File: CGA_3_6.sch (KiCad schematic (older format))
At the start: 1 part, among them U4 74S174

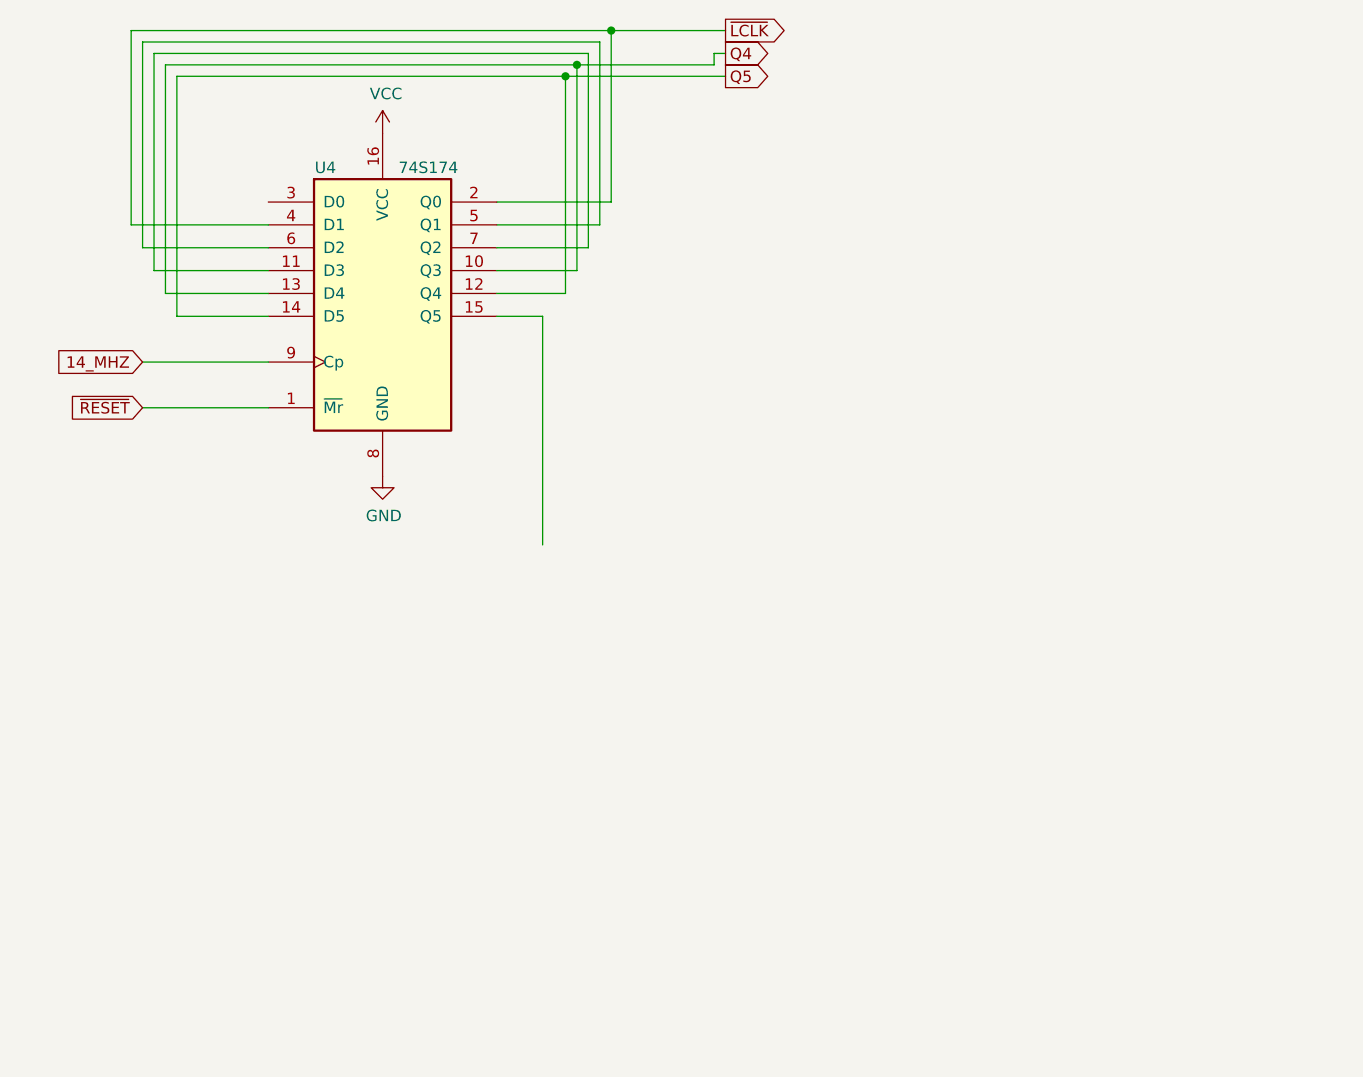
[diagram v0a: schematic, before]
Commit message: More sheet 3 drawing
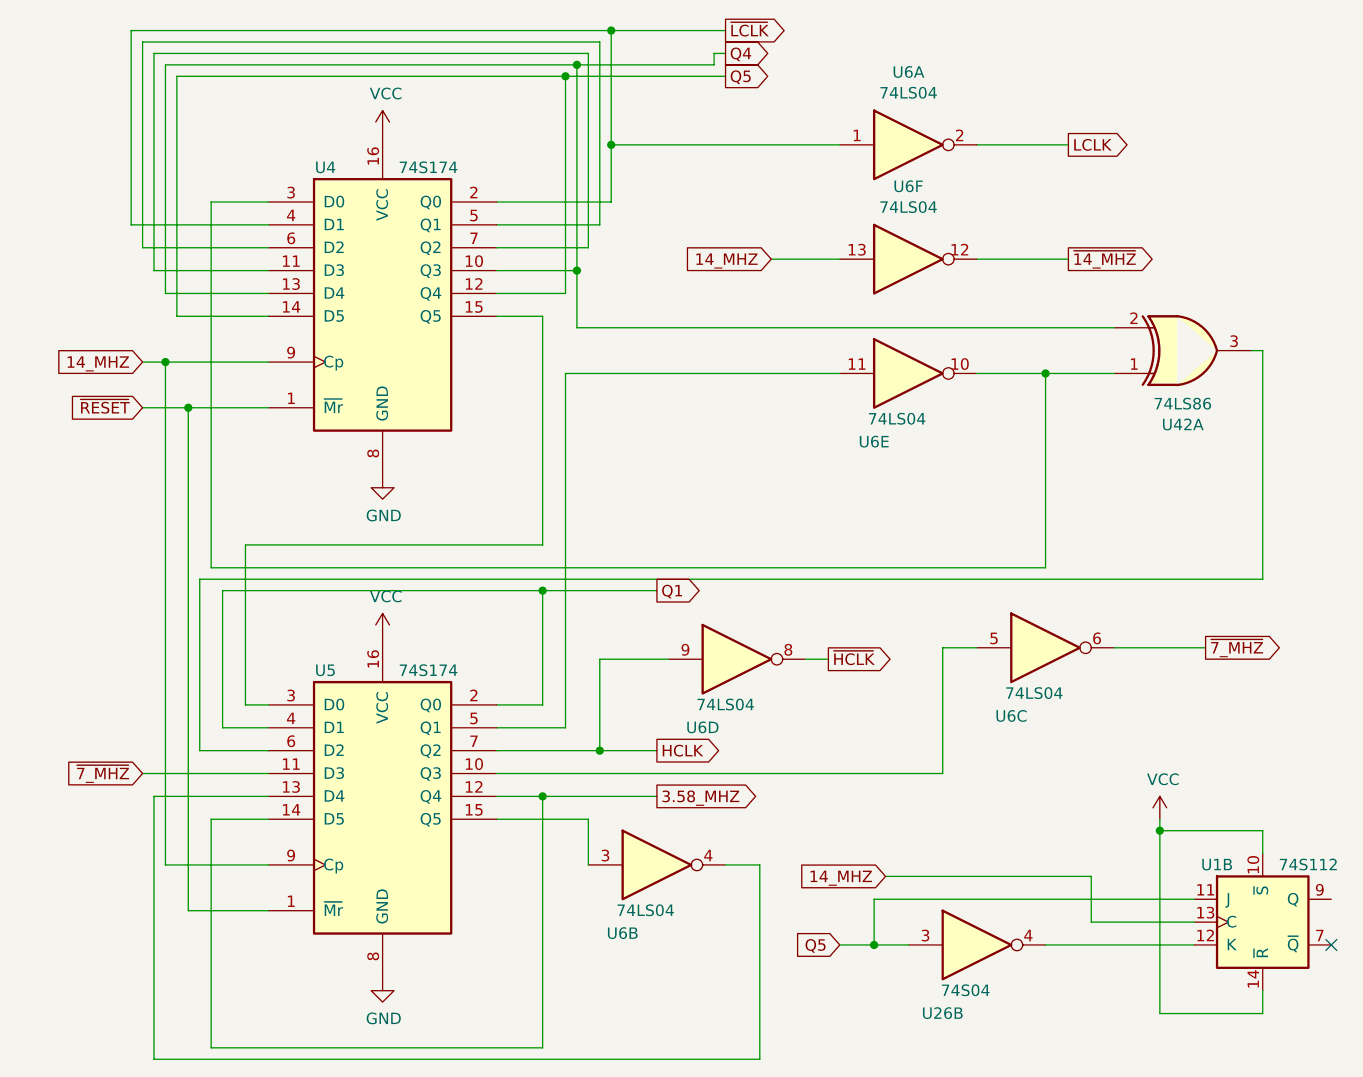
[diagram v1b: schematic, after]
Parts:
- added U1: 74S112, Package_DIP:DIP-16_W7.62mm_LongPads, symbol 74xx:74LS112
- added U26: 74S04, Package_DIP:DIP-14_W7.62mm_LongPads, symbol 74xx:74LS04
- added U42: 74LS86, Package_DIP:DIP-14_W7.62mm_LongPads, symbol 74xx:74LS86
- added U5: 74S174, Package_DIP:DIP-16_W7.62mm_LongPads, symbol 74xx:74LS174
- added U6: 74LS04, Package_DIP:DIP-14_W7.62mm_LongPads, symbol 74xx:74LS04
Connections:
- net labels added: 3.58_MHZ, HCLK, LCLK, Q1, ~14_MHZ, ~7_MHZ, ~HCLK
- wire segments 34 -> 107
- no-connect marks 0 -> 1
